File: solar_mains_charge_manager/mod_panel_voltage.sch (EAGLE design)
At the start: 31 parts, among them IC1 ACS750LCA-050, T1 TIP122, X10 22-23-2041, X2 22-23-2021, X3 22-23-2031, X5 22-23-2031, X6 22-23-2041, X7 53047-15, X8 53047-15

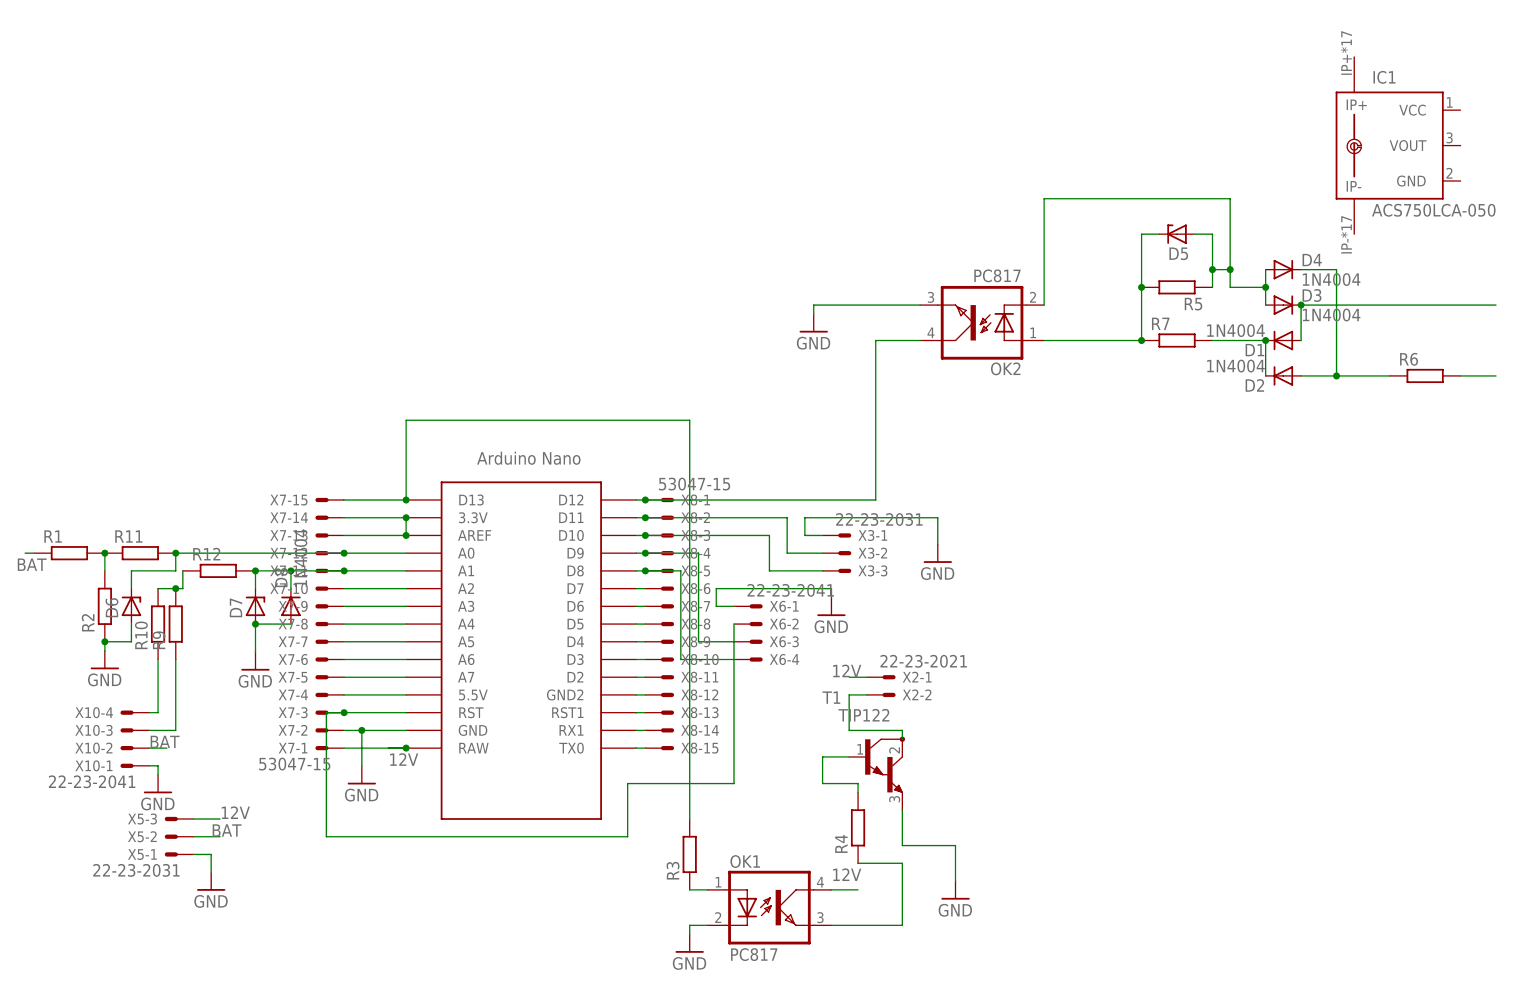
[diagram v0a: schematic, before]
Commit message: A lot of stuff
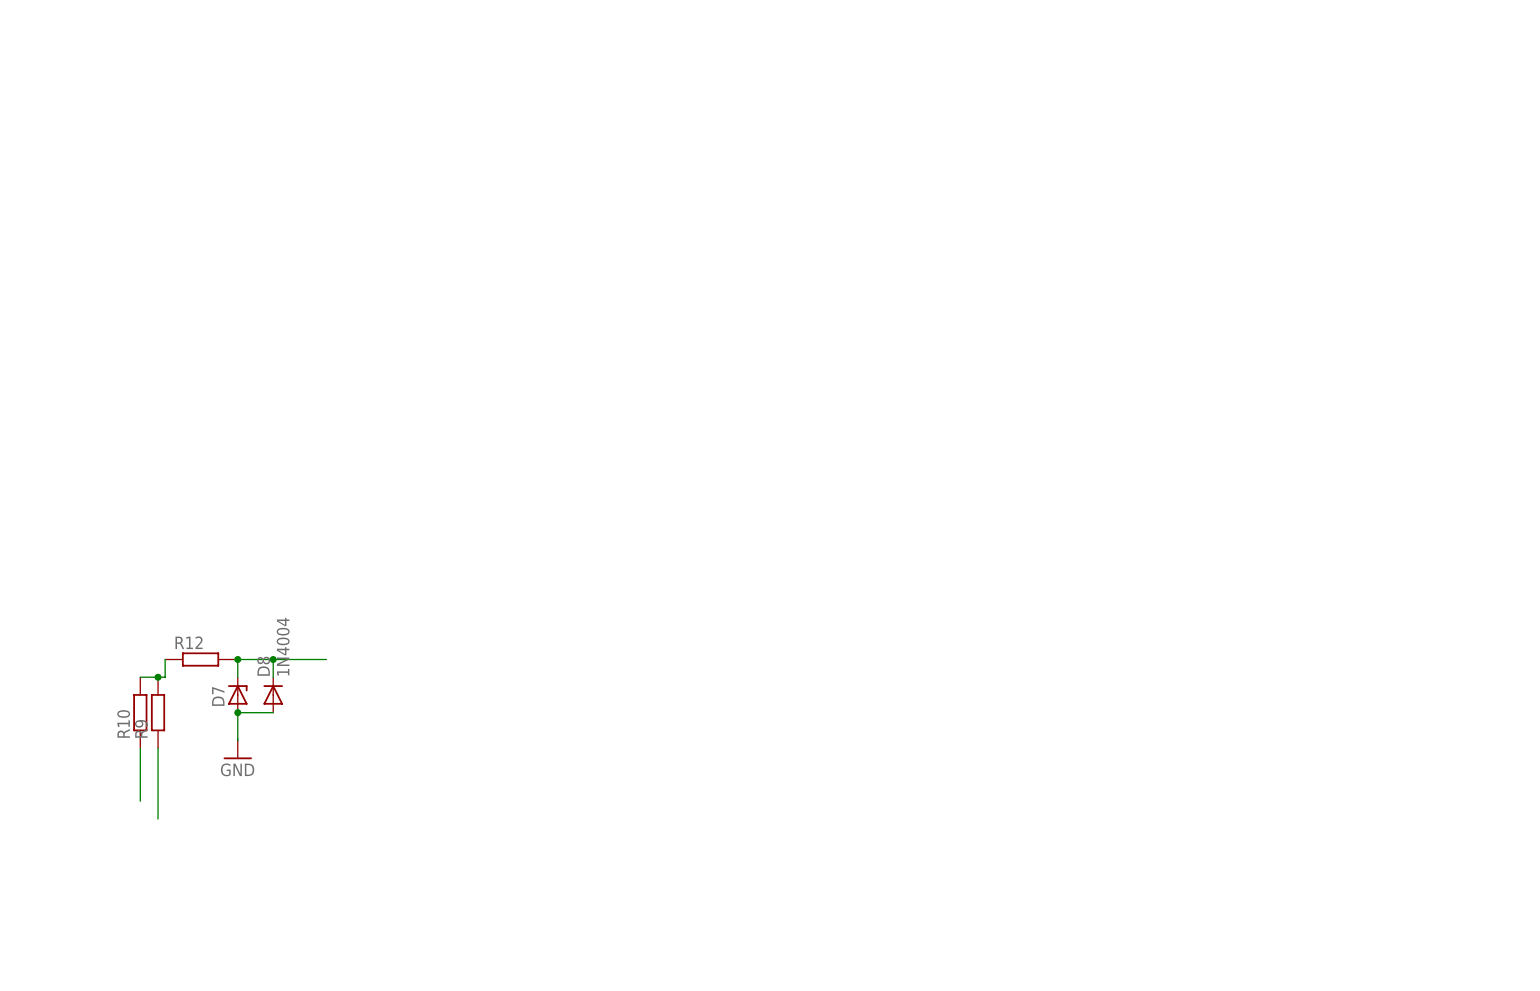
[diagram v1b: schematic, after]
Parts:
- removed D1, D2, D3, D4: 1N4004, diode:1N4004
- removed D5, D6: (no value), diode:ZENER-DIODEDO34-7
- removed IC1: ACS750LCA-050, allegro:ACS750LCA-050
- removed OK1, OK2: PC817, optocoupler:PC817
- removed R1, R11, R2, R3, R4, R5: (no value), resistor:R-EU_0204/5
- removed R6, R7: (no value), resistor:R-EU_0204/7
- removed T1: TIP122, transistor:TIP122
- removed U$1: NANO, Arduino-clone:NANO
- removed X10, X6: 22-23-2041, con-molex:22-23-2041
- removed X2: 22-23-2021, con-molex:22-23-2021
- removed X3, X5: 22-23-2031, con-molex:22-23-2031
- removed X7, X8: 53047-15, con-molex:53047-15
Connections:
- removed net 12V: OK1.COL, U$1.RAW, X2-1.S, X5-3.S, X7-1.S
- removed net BAT: R1.1, X10-2.S, X5-2.S
- removed net N$1: U$1.3.3V, U$1.AREF, X7-13.S, X7-14.S
- removed net N$11: D1.C, D2.C, R7.2
- removed net N$12: OK2.COL, U$1.D12, X8-1.S
- removed net N$13: D1.A, D3.C
- removed net N$15: D2.A, D4.C, R6.1
- removed net N$16: R6.2
- removed net N$17: U$1.D11, X3-2.S, X8-2.S
- removed net N$18: U$1.D10, X3-3.S, X8-3.S
- removed net N$19: U$1.D9, X6-3.S, X8-4.S
- removed net N$2: R3.2, U$1.D13, X7-15.S
- removed net N$20: U$1.D8, X6-4.S, X8-5.S
- removed net N$21: U$1.RST, X6-2.S, X7-3.S
- removed net N$22: U$1.D7, X8-6.S
- removed net N$23: U$1.D6, X8-7.S
- removed net N$24: U$1.D5, X8-8.S
- removed net N$25: U$1.D4, X8-9.S
- removed net N$26: U$1.D3, X8-10.S
- removed net N$27: U$1.D2, X8-11.S
- removed net N$28: U$1.GND2, X8-12.S
- removed net N$29: U$1.RST1, X8-13.S
- removed net N$30: U$1.RX1, X8-14.S
- removed net N$31: U$1.TX0, X8-15.S
- removed net N$32: U$1.5.5V, X7-4.S
- removed net N$33: U$1.A7, X7-5.S
- removed net N$34: U$1.A6, X7-6.S
- removed net N$35: U$1.A5, X7-7.S
- removed net N$36: U$1.A4, X7-8.S
- removed net N$37: U$1.A3, X7-9.S
- removed net N$38: U$1.A2, X7-10.S
- removed net N$4: OK1.A, R3.1
- removed net N$40: D6.C, R11.2, U$1.A0, X7-12.S
- removed net N$43: R1.2, R11.1, R2.2
- removed net N$5: T1.C, X2-2.S
- removed net N$6: OK1.EMIT, R4.1
- removed net N$7: R4.2, T1.B
- removed net N$8: D3.A, D4.A, D5.A, OK2.C, R5.1
- removed net N$9: D5.C, OK2.A, R5.2, R7.1
- net GND: no longer D6.A, OK1.C, OK2.EMIT, R2.1, T1.E, U$1.GND, X10-1.S, X3-1.S, X5-1.S, X6-1.S, X7-2.S
- net N$39: no longer U$1.A1, X7-11.S
- net N$41: no longer X10-4.S
- net N$42: no longer X10-3.S
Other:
- moved on the sheet: D7, D8, R10, R12, R9
